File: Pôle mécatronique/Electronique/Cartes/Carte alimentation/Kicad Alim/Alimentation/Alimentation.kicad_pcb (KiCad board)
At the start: 2 copper layers, 68.6 x 78.7 mm, 22 parts, among them J1 Conn_01x04, J2 Conn_01x04, J3 Conn_01x04, J4 Conn_01x05, J5 Conn_01x05, J6 Conn_02x03_Odd_Even, J7 Conn_02x10_Odd_Even, J8 Conn_01x02, J9 Conn_01x02, K1 G5LE-1, Q1 BD135, U1 TSR_2-2450, U2 TSR_2-2450, U3 TSR_2-24120

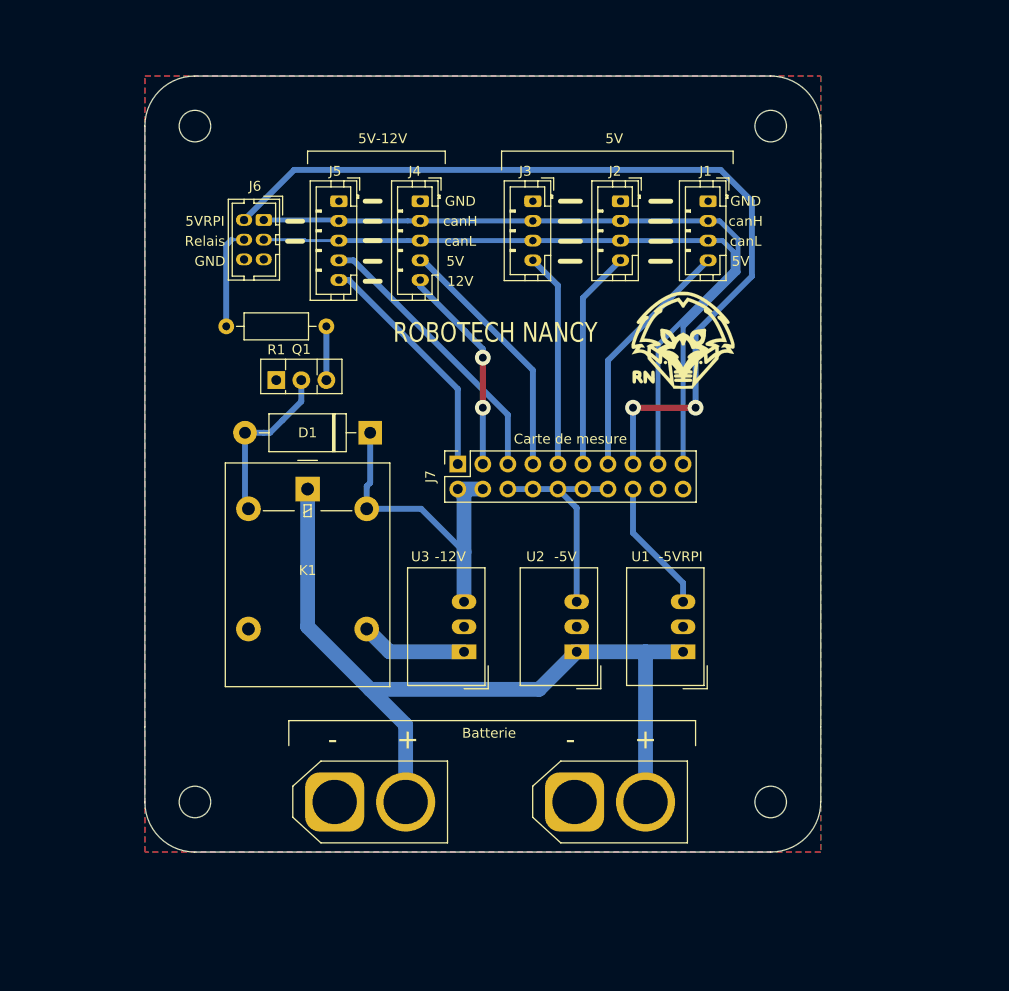
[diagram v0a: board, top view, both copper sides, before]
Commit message: Update alim sécurité
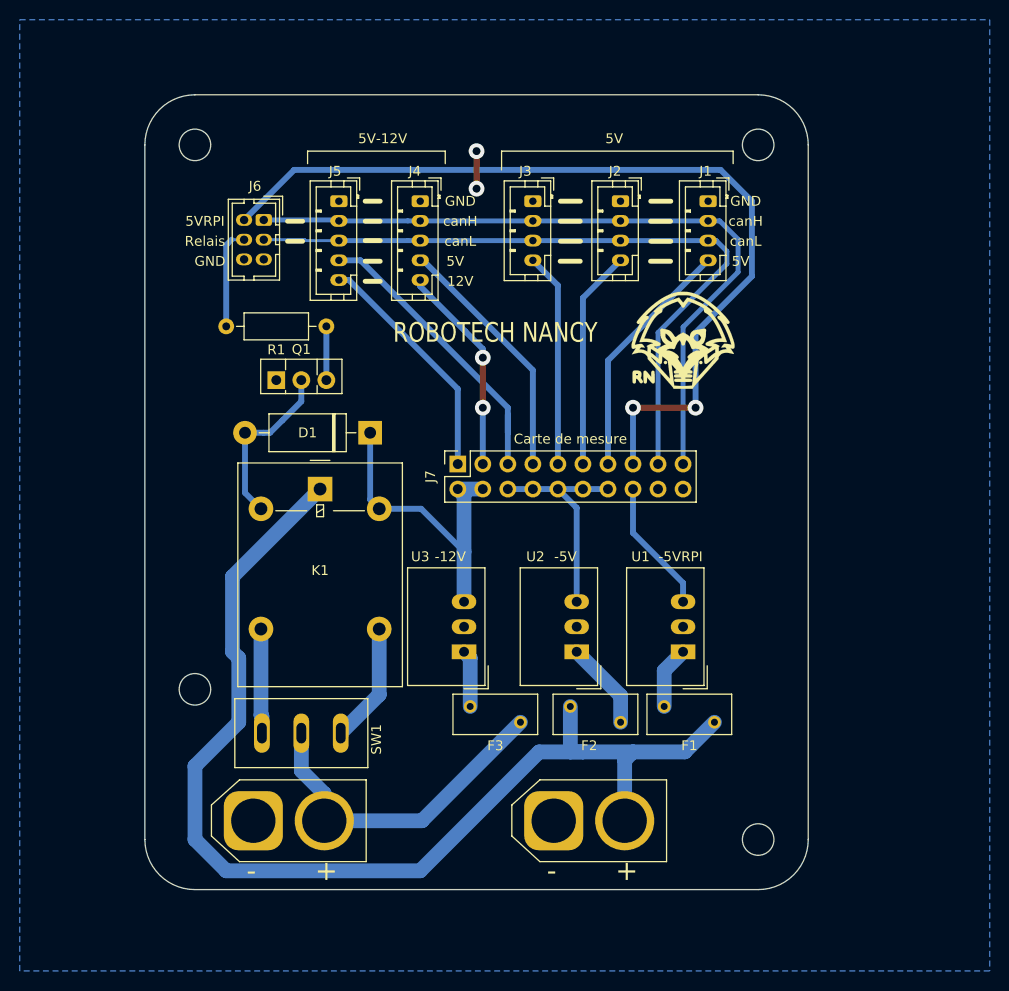
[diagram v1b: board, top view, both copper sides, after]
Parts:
- added F1: 2A, Fuse:Fuse_BelFuse_0ZRE0012FF_L8.3mm_W3.8mm, F.Cu at (138.5, 97.5)
- added F2: 2A, Fuse:Fuse_BelFuse_0ZRE0012FF_L8.3mm_W3.8mm, F.Cu at (134.1, 99.1)
- added F3: 2A, Fuse:Fuse_BelFuse_0ZRE0012FF_L8.3mm_W3.8mm, F.Cu at (118.9, 97.5)
- added SW1: SW_DPDT_x2, Autre:Switch_3_Pin, F.Cu at (101.7, 100.2)
- J8: value Conn_01x02 -> 24V in
- J9: value Conn_01x02 -> 24V out
- moved J9 32.7 mm to (96.9, 109.1)
- moved J8 22.3 mm to (127.3, 109.1)
- moved REF** 11.4 mm to (90.9, 95.8)
- moved REF** 4.02 mm to (148.1, 111.0)
- moved REF** 2.29 mm to (148.1, 40.5)
- moved REF** 1.91 mm to (90.9, 40.5)
- moved K1 1.27 mm to (103.6, 75.4)
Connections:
- J9 pad 2: Vbatt -> VbattRelay
- K1 pad 3: unconnected-(K1-Pad3) -> Net-(K1-Pad3)
- K1 pad 4: VbattProtected -> Net-(K1-Pad4)
- U1 pad 1: Vbatt -> Net-(U1-Pad1)
- U2 pad 1: Vbatt -> Net-(U2-Pad1)
- U3 pad 1: VbattProtected -> Net-(U3-Pad1)
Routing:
- net VbattRelay: track 0.00 -> 33.9 mm
- net Vbatt: track 84.8 -> 114.8 mm
- net Net-(K1-Pad4): track 0.00 -> 12.2 mm
- net VbattProtected: track 10.8 -> 0.00 mm
- net Net-(K1-Pad3): track 0.00 -> 10.6 mm
- net Net-(U2-Pad1): track 0.00 -> 9.00 mm
- net Net-(U1-Pad1): track 0.00 -> 6.34 mm
- net Net-(U3-Pad1): track 0.00 -> 5.81 mm
- net GND: track 0.00 -> 3.81 mm, vias 0 -> 2
- net 5Vout5: track 28.6 -> 30.9 mm
- net 12V: track 34.3 -> 32.7 mm
- net can_L: track 73.5 -> 72.6 mm
- net Net-(D1-Pad2): track 17.1 -> 17.6 mm
- removed copper zone on F.Cu, net GND
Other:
- board size 68.6 x 78.7 mm -> 67.3 x 80.6 mm
- board text removed: "Batterie"
